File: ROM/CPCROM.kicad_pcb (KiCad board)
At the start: 2 copper layers, 99.1 x 49.9 mm, 27 parts, among them IC103 SST39SF040, IC190 74LS374, IC191 74LS32, IC192 74LS32, IC193 74LS02, IC194 74LS08, IC195 74LS74

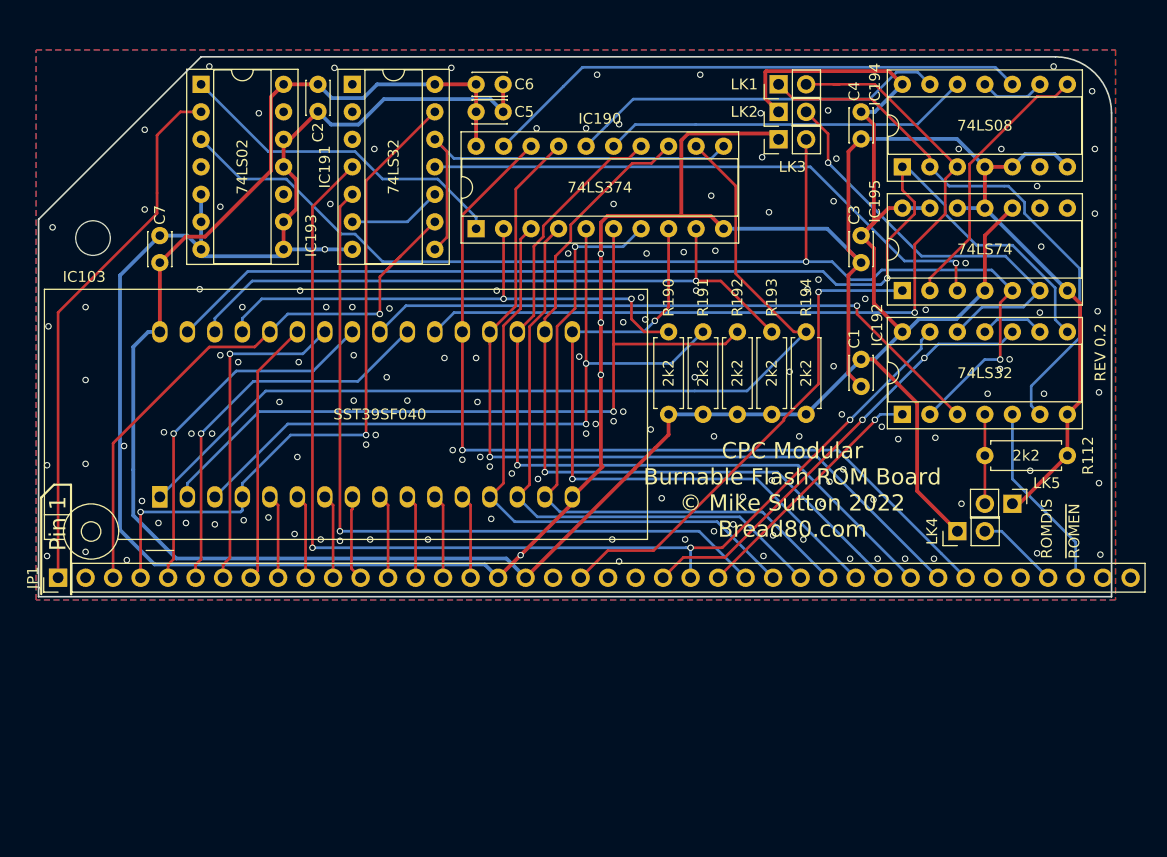
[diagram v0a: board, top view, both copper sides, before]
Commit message: Long overdue update...
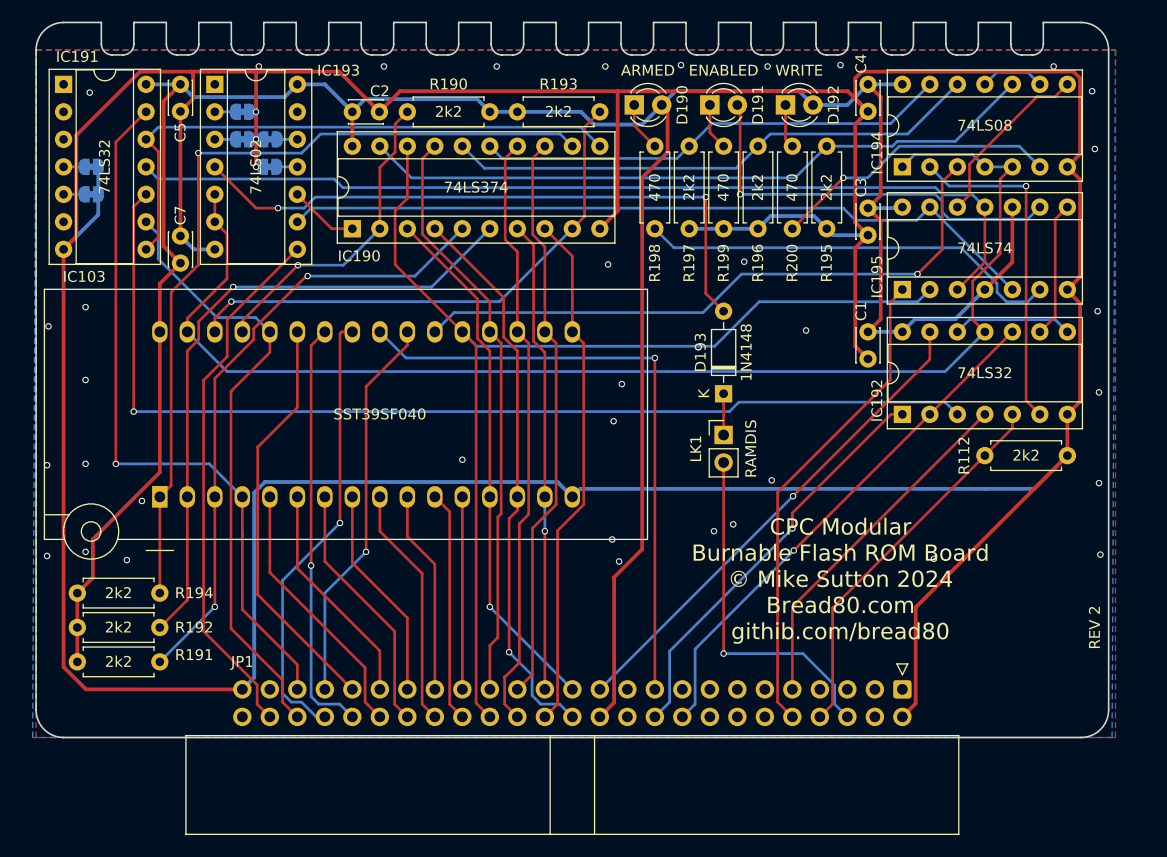
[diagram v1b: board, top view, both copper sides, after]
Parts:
- removed ?: , Mounting_Holes:MountingHole_3.2mm_M3
- removed C6: 0.1nF, Capacitor_THT:C_Disc_D3.0mm_W2.0mm_P2.50mm
- removed LK2, LK3, LK4, LK5: Jumper_NO_Small, Connector_PinHeader_2.54mm:PinHeader_1x02_P2.54mm_Vertical
- added D190: ARMED, LED_THT:LED_D3.0mm, F.Cu at (208.9, 108.0)
- added D191: ENABLED, LED_THT:LED_D3.0mm, F.Cu at (215.9, 108.0)
- added D192: WRITE, LED_THT:LED_D3.0mm, F.Cu at (222.9, 108.0)
- added D193: 1N4148, Diode_THT:D_DO-35_SOD27_P7.62mm_Horizontal, F.Cu at (217.2, 134.6)
- added JP2: Jumper_NC_Small, Jumper:SolderJumper-2_P1.3mm_Bridged_RoundedPad1.0x1.5mm, B.Cu at (175.2, 113.7)
- added JP3: Jumper_NC_Small, Jumper:SolderJumper-2_P1.3mm_Bridged_RoundedPad1.0x1.5mm, B.Cu at (175.3, 111.1)
- added JP4: Jumper_NC_Small, Jumper:SolderJumper-2_P1.3mm_Bridged_RoundedPad1.0x1.5mm, B.Cu at (172.7, 108.6)
- added JP5: Jumper_NC_Small, Jumper:SolderJumper-2_P1.3mm_Bridged_RoundedPad1.0x1.5mm, B.Cu at (172.7, 111.1)
- added JP6: Jumper_NC_Small, Jumper:SolderJumper-2_P1.3mm_Bridged_RoundedPad1.0x1.5mm, B.Cu at (158.8, 113.7)
- added JP7: Jumper_NC_Small, Jumper:SolderJumper-2_P1.3mm_Bridged_RoundedPad1.0x1.5mm, B.Cu at (158.8, 116.2)
- added R195: 2k2, Resistor_THT:R_Axial_DIN0207_L6.3mm_D2.5mm_P7.62mm_Horizontal, F.Cu at (226.7, 119.4)
- added R196: 2k2, Resistor_THT:R_Axial_DIN0207_L6.3mm_D2.5mm_P7.62mm_Horizontal, F.Cu at (220.3, 119.4)
- added R197: 2k2, Resistor_THT:R_Axial_DIN0207_L6.3mm_D2.5mm_P7.62mm_Horizontal, F.Cu at (214.0, 119.4)
- added R198: 470, Resistor_THT:R_Axial_DIN0207_L6.3mm_D2.5mm_P7.62mm_Horizontal, F.Cu at (210.8, 111.8)
- added R199: 470, Resistor_THT:R_Axial_DIN0207_L6.3mm_D2.5mm_P7.62mm_Horizontal, F.Cu at (217.2, 111.8)
- added R200: 470, Resistor_THT:R_Axial_DIN0207_L6.3mm_D2.5mm_P7.62mm_Horizontal, F.Cu at (223.5, 111.8)
- JP1: value RC2014Bus -> Conn_02x25_Odd_Even; footprint Connector_PinHeader_2.54mm:PinHeader_1x40_P2.54mm_Vertical -> Connector_IDC:IDC-Header_2x25_P2.54mm_Horizontal
- LK1: value Jumper_NO_Small -> RAMDIS
- moved JP1 78.7 mm to (233.7, 161.9), turned to 270 degrees
- moved R194 69.3 mm to (157.5, 153.0), turned to 0 degrees
- moved R192 64.1 mm to (157.5, 156.2), turned to 0 degrees
- moved R191 62.1 mm to (157.5, 159.4), turned to 0 degrees
- moved R193 36.5 mm to (198.1, 108.6), turned to 0 degrees
- moved LK1 32.8 mm to (217.2, 138.4), turned to 0 degrees
- moved R190 32.5 mm to (195.6, 108.6), turned to 180 degrees
- moved C5 27.4 mm to (167.0, 106.0), turned to 270 degrees
- moved IC191 26.7 mm to (156.2, 106.0)
- moved IC190 11.4 mm to (182.9, 119.4)
- moved C2 4.07 mm to (182.9, 108.6), turned to 0 degrees
- moved C3 2.62 mm to (230.5, 117.5)
- moved C1 2.62 mm to (230.5, 128.9)
- moved C4 2.62 mm to (230.5, 106.0)
- moved C7 1.91 mm to (167.0, 122.6)
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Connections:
- IC103 pad 24: Net-(IC103-Pad24) -> /~RD
- IC103 pad 31: Net-(IC103-Pad31) -> WRITE
- IC191 pad 4: /ROM/~WR -> Net-(IC191-Pad4)
- IC191 pad 5: /ROM/~IORQ -> Net-(IC191-Pad5)
- IC191 pad 6: Net-(IC191-Pad10) -> Net-(IC191-Pad6)
- IC192 pad 1: /ROM/~RD -> /~IORQ
- IC192 pad 10: /ROM/~MREQ -> /~WR
- IC192 pad 11: Net-(IC192-Pad11) -> WRITE
- IC192 pad 12: /ROM/~WRITE_EN -> Net-(IC192-Pad12)
- IC192 pad 13: /ROM/~WR -> /~MREQ
- IC192 pad 2: /ROM/WRITE_EN -> /~WR
- IC192 pad 3: Net-(IC103-Pad24) -> Net-(IC191-Pad10)
- IC192 pad 4: Net-(IC192-Pad4) -> /~ROMEN
- IC192 pad 5: /ROM/~ROMEN -> /ROMDIS
- IC192 pad 8: Net-(IC103-Pad31) -> Net-(IC192-Pad12)
- IC192 pad 9: Net-(IC192-Pad11) -> /ROM/~WRITE_EN
- IC193 pad 1: Net-(IC190-Pad1) -> Net-(IC193-Pad1)
- IC193 pad 10: Net-(IC193-Pad10) -> Net-(IC190-Pad1)
- IC193 pad 11: GND -> Net-(IC193-Pad11)
- IC193 pad 12: GND -> Net-(IC193-Pad12)
- IC193 pad 2: A15 -> Net-(IC193-Pad2)
- IC193 pad 3: /ROM/WRITE_EN -> Net-(IC193-Pad3)
- IC193 pad 5: GND -> WRITE
- IC193 pad 6: GND -> WRITE
- IC193 pad 8: GND -> A15
- IC193 pad 9: GND -> /ROM/ARMED
- IC194 pad 1: Net-(IC103-Pad31) -> WRITE
- IC194 pad 12: Net-(IC190-Pad15) -> Net-(IC190-Pad16)
- IC194 pad 13: Net-(IC190-Pad16) -> Net-(IC190-Pad15)
- IC194 pad 4: GND -> WRITE
- IC194 pad 5: GND -> WRITE
- IC195 pad 1: /ROM/~RESET -> /~RESET
- IC195 pad 11: GND -> Net-(IC191-Pad11)
- IC195 pad 12: GND -> Net-(IC194-Pad8)
- IC195 pad 13: +5V -> /ROM/ARMED
- IC195 pad 2: Net-(IC194-Pad8) -> D7
- IC195 pad 5: /ROM/WRITE_EN -> /ROM/ARMED
- IC195 pad 6: /ROM/~WRITE_EN -> ~ARMED
- IC195 pad 8: Net-(IC195-Pad8) -> /ROM/~WRITE_EN
- IC195 pad 9: Net-(IC195-Pad9) -> WRITE_EN
- JP1 pad 1: A15 -> Net-(JP1-Pad1)
- JP1 pad 10: A6 -> /~RESET
- JP1 pad 11: A5 -> Net-(JP1-Pad11)
- JP1 pad 12: A4 -> Net-(JP1-Pad12)
- JP1 pad 13: A3 -> Net-(JP1-Pad13)
- JP1 pad 14: A2 -> Net-(JP1-Pad14)
- JP1 pad 15: A1 -> Net-(JP1-Pad15)
- JP1 pad 16: A0 -> Net-(JP1-Pad16)
- JP1 pad 17: GND -> Net-(JP1-Pad17)
- JP1 pad 18: +5V -> /~WR
- JP1 pad 19: Net-(JP1-Pad19) -> /~RD
- JP1 pad 2: A14 -> GND
- JP1 pad 20: /ROM/~RESET -> /~IORQ
- JP1 pad 23: /ROM/~MREQ -> /~MREQ
- JP1 pad 24: /ROM/~WR -> +5V
- JP1 pad 25: /ROM/~RD -> D0
- JP1 pad 26: /ROM/~IORQ -> D1
- JP1 pad 27: D0 -> D2
- JP1 pad 28: D1 -> D3
- JP1 pad 29: D2 -> D4
- JP1 pad 3: A13 -> Net-(JP1-Pad3)
- JP1 pad 30: D3 -> D5
- JP1 pad 31: D4 -> D6
- JP1 pad 32: D5 -> D7
- JP1 pad 33: D6 -> A0
- JP1 pad 34: D7 -> A1
- JP1 pad 35: Net-(JP1-Pad35) -> A2
- JP1 pad 36: Net-(JP1-Pad36) -> A3
- JP1 pad 37: /ROM/ROMDIS -> A4
- JP1 pad 38: /ROM/~ROMEN -> A5
- JP1 pad 39: Net-(JP1-Pad39) -> A6
- JP1 pad 4: A12 -> Net-(JP1-Pad4)
- JP1 pad 40: Net-(JP1-Pad40) -> A7
- JP1 pad 5: A11 -> Net-(JP1-Pad5)
- JP1 pad 6: A10 -> /RAMDIS
- JP1 pad 7: A9 -> Net-(JP1-Pad7)
- JP1 pad 8: A8 -> /ROMDIS
- JP1 pad 9: A7 -> /~ROMEN
- LK1 pad 1: Net-(IC192-Pad6) -> Net-(D193-Pad1)
- LK1 pad 2: Net-(IC103-Pad22) -> /RAMDIS
- R112 pad 1: Net-(IC192-Pad4) -> /ROMDIS
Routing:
- net GND: track 291.4 -> 427.5 mm, vias 144 -> 39
- net WRITE: track 0.00 -> 119.7 mm
- net /ROM/WRITE_EN: track 108.2 -> 0.00 mm, vias 2 -> 0
- net /ROM/~WR: track 105.2 -> 0.00 mm, vias 3 -> 0
- net Net-(IC103-Pad31): track 103.2 -> 0.00 mm, vias 1 -> 0
- net Net-(IC191-Pad10): track 8.67 -> 97.4 mm, vias 0 -> 1
- net /ROM/~IORQ: track 70.8 -> 0.00 mm, vias 1 -> 0
- net /ROM/ARMED: track 0.00 -> 70.7 mm
- net Net-(IC103-Pad24): track 58.9 -> 0.00 mm, vias 1 -> 0
- net Net-(D193-Pad2): track 0.00 -> 58.6 mm, vias 0 -> 2
- net /~RD: track 0.00 -> 57.0 mm, vias 0 -> 1
- net /~WR: track 0.00 -> 48.2 mm, vias 0 -> 1
- net /ROM/~RESET: track 45.8 -> 0.00 mm, vias 1 -> 0
- net /~MREQ: track 0.00 -> 45.6 mm, vias 0 -> 1
- net /~RESET: track 0.00 -> 44.7 mm
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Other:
- board size 99.1 x 49.9 mm -> 99.1 x 66 mm
- board text added: "All capacitors are 100nF unless marked. LEDs are 3mm, your choice of colours. JP1 is MX4 compatible."
- board text added: "CPC Modular Burnable Flash ROM Board © Mike Sutton 2024 Bread80.com githib.com/bread80"
- board text added: "HOW TO FLASH THE EEPROM out (&cfff),ROM_number OR $e0 ;Arm <repeat above instruction> ;Write enable <Program FLASH as per datasheet> out (&cfff),ROM_number ;Disable and disarm When write enabled: * A15 and A14 are ignored. * The flash maps to *all* memory banks. * Writes to RAM are disbled (if LK1 installed). * Firmware is in bank 31. ROM burning code *must* run from RAM. Interrupts *must* be dis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"
- board text added: "REV 2"
- board text added: "ROM slot 31 is firmware Slots 0..30 are upper ROMs Ports: ROM select: &dfff. Write control: &cfff"
- board text added: "Short LK1 to output RAMDIS while writing to flash. (You want to do this, unless there's a bug)."
- board text removed: "CPC Modular Burnable Flash ROM Board for RC2014 Backplanes © Mike Sutton 2022 Bread80.com"
- board text removed: "CPC Modular Burnable Flash ROM Board © Mike Sutton 2022 Bread80.com"
- board text removed: "For CPC (ROM override) install LK4 and LK5. For CPC modular install link across LK4 to LK5 round holes."
- board text removed: "Pin 1"
- board text removed: "REV 0.2"
- board text removed: "ROMDIS"
- board text removed: "To enable writing, install IC194 & IC195 and leave LK1, LK2, LK3 empty. If installing the links the ICs listed above **must** be removed."
- board text removed: "~ROMEN"
